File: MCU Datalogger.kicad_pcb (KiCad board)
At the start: 2 copper layers, 29 parts, among them J1 Conn_01x04_Pin, J2 Conn_01x04_Pin, J3 Conn_01x09_Pin, J4 Conn_02x03_Odd_Even, U1 24LC1025, U2 24LC1025, U3 DS1337S_, U4 ATMEGA328P-AU, Y1 32.768 KHz, Y2 16 MHz

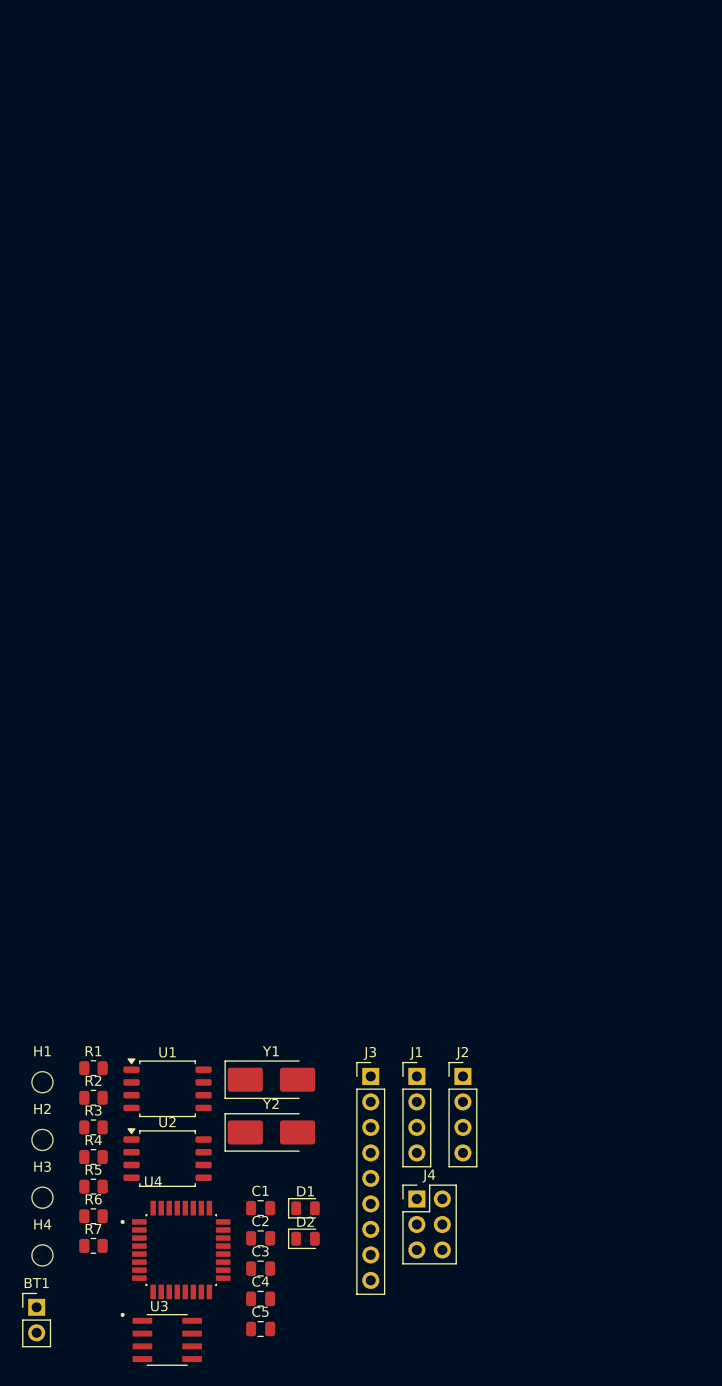
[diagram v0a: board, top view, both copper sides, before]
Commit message: Completed placements of footprints.
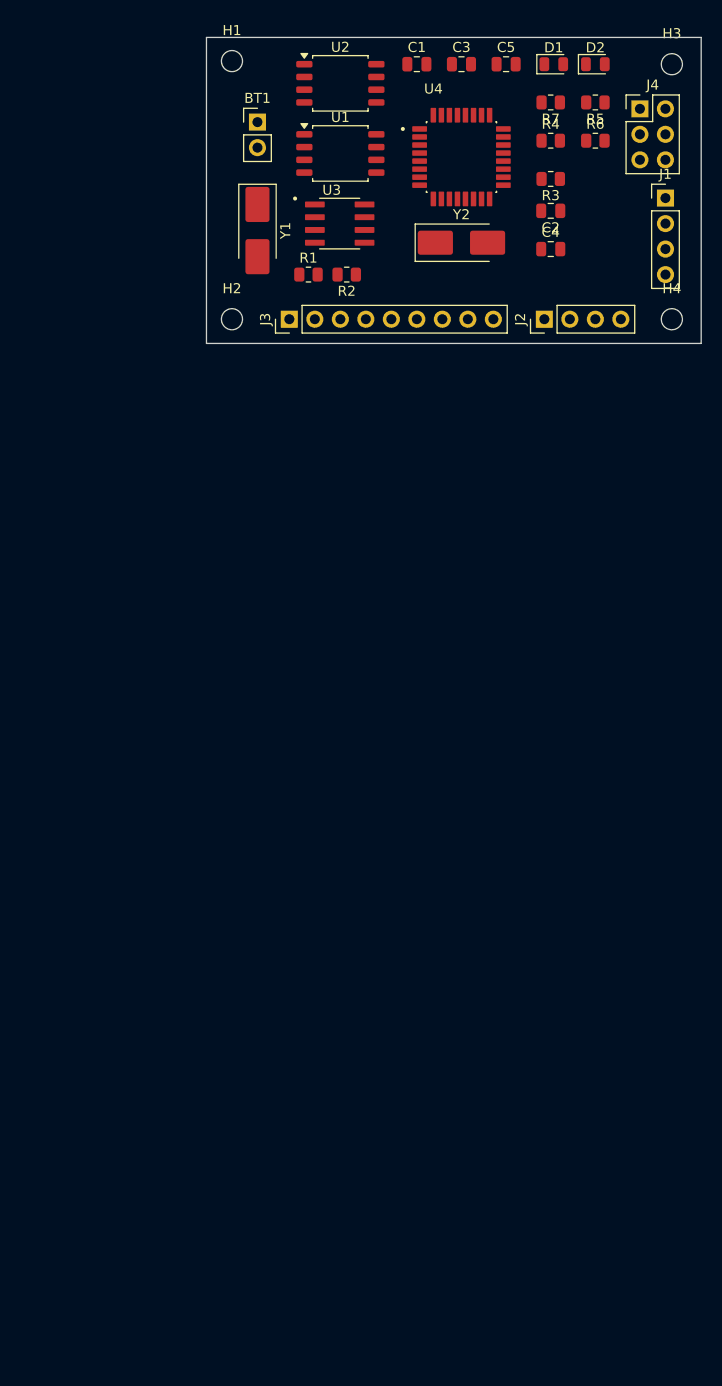
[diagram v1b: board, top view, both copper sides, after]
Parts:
- moved H3 129.1 mm to (110.5, 38.1)
- moved C5 128.3 mm to (94.0, 38.1)
- moved R7 122.7 mm to (98.4, 41.9), turned to 180 degrees
- moved C3 121.6 mm to (89.5, 38.1)
- moved D2 120.5 mm to (102.9, 38.1)
- moved BT1 120.1 mm to (69.2, 43.9)
- moved R5 119.0 mm to (102.9, 41.9), turned to 180 degrees
- moved R6 118.2 mm to (102.9, 45.7)
- moved D1 116.6 mm to (98.7, 38.1)
- moved C1 115.0 mm to (85.1, 38.1)
- moved U3 112.5 mm to (77.4, 54.0)
- moved U4 112.4 mm to (89.5, 47.4)
- moved H4 112.4 mm to (110.5, 63.5)
- moved R4 111.0 mm to (98.4, 45.7)
- moved J4 110.8 mm to (107.3, 42.5)
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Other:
- board outline added: 49.3 x 30.5 mm
